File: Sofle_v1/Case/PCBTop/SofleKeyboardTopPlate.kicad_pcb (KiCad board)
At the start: 2 copper layers, 137.2 x 109.2 mm, 5 parts

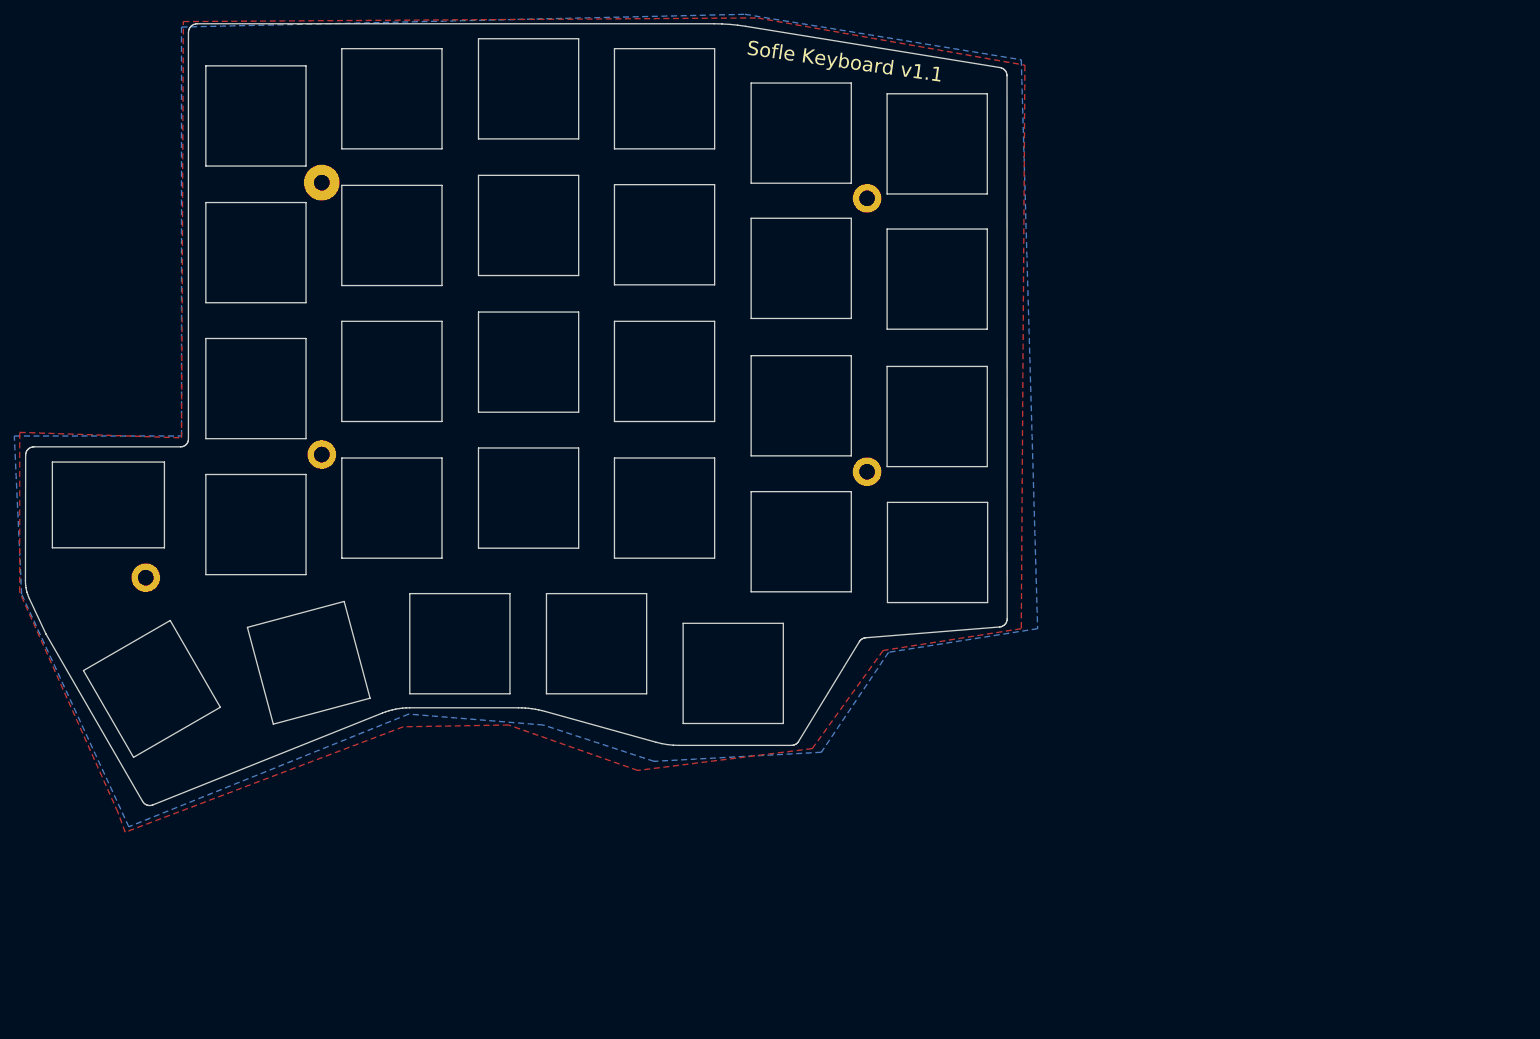
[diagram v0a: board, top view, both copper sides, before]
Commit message: Plates.
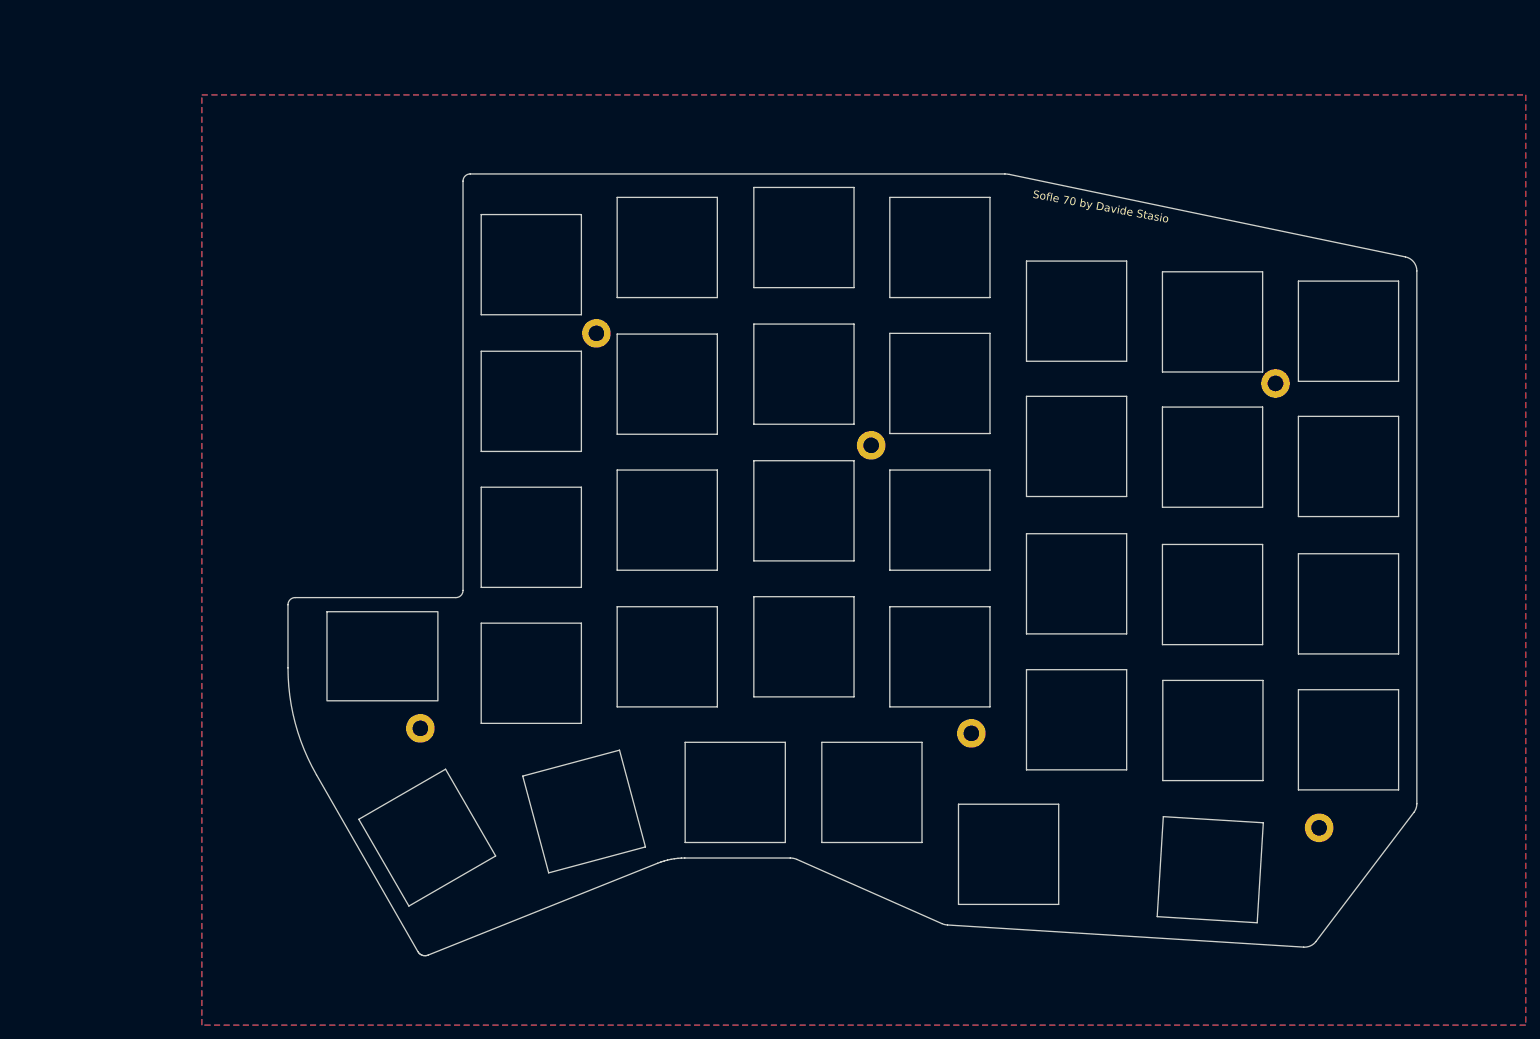
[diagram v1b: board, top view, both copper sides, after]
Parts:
- removed ? (x5): , Wire_Pads:SolderWirePad_single_0-8mmDrill
- added SW1: SW_PUSH, SofleKeyboard:CherryMX_KailhLowProfile_Hotswap_Top-Plate, F.Cu at (91.0, 50.2)
- added SW10: SW_PUSH, SofleKeyboard:CherryMX_KailhLowProfile_Hotswap_Top-Plate, F.Cu at (148.1, 66.8)
- added SW11: SW_PUSH, SofleKeyboard:CherryMX_KailhLowProfile_Hotswap_Top-Plate, F.Cu at (167.2, 75.6)
- added SW12: SW_PUSH, SofleKeyboard:CherryMX_KailhLowProfile_Hotswap_Top-Plate, F.Cu at (186.2, 77.1)
- added SW13: SW_PUSH, SofleKeyboard:CherryMX_KailhLowProfile_Hotswap_Top-Plate, F.Cu at (91.0, 88.3)
- added SW14: SW_PUSH, SofleKeyboard:CherryMX_KailhLowProfile_Hotswap_Top-Plate, F.Cu at (110.0, 85.9)
- added SW15: SW_PUSH, SofleKeyboard:CherryMX_KailhLowProfile_Hotswap_Top-Plate, F.Cu at (129.1, 84.6)
- added SW16: SW_PUSH, SofleKeyboard:CherryMX_KailhLowProfile_Hotswap_Top-Plate, F.Cu at (148.1, 85.9)
- added SW17: SW_PUSH, SofleKeyboard:CherryMX_KailhLowProfile_Hotswap_Top-Plate, F.Cu at (167.2, 94.8)
- added SW18: SW_PUSH, SofleKeyboard:CherryMX_KailhLowProfile_Hotswap_Top-Plate, F.Cu at (186.2, 96.3)
- added SW19: SW_PUSH, SofleKeyboard:CherryMX_KailhLowProfile_Hotswap_Top-Plate, F.Cu at (91.0, 107.3)
- added SW2: SW_PUSH, SofleKeyboard:CherryMX_KailhLowProfile_Hotswap_Top-Plate, F.Cu at (110.0, 47.8)
- added SW20: SW_PUSH, SofleKeyboard:CherryMX_KailhLowProfile_Hotswap_Top-Plate, F.Cu at (110.0, 105.0)
- added SW21: SW_PUSH, SofleKeyboard:CherryMX_KailhLowProfile_Hotswap_Top-Plate, F.Cu at (129.1, 103.6)
- added SW22: SW_PUSH, SofleKeyboard:CherryMX_KailhLowProfile_Hotswap_Top-Plate, F.Cu at (148.1, 105.0)
- added SW23: SW_PUSH, SofleKeyboard:CherryMX_KailhLowProfile_Hotswap_Top-Plate, F.Cu at (167.2, 113.8)
- added SW24: SW_PUSH, SofleKeyboard:CherryMX_KailhLowProfile_Hotswap_Top-Plate, F.Cu at (186.3, 115.3)
- added SW25: Rotary_Encoder_Switch, SofleKeyboard:RotaryEncoder_Alps_EC11E-Switch_Vertical_H20mm-keebio_Top-Plate, F.Cu at (70.5, 104.7)
- added SW26: SW_PUSH, SofleKeyboard:CherryMX_KailhLowProfile_Hotswap_Top-Plate, F.Cu at (76.5, 130.3)
- added SW27: SW_PUSH, SofleKeyboard:CherryMX_KailhLowProfile_Hotswap_Top-Plate, F.Cu at (98.4, 126.6)
- added SW28: SW_PUSH, SofleKeyboard:CherryMX_KailhLowProfile_Hotswap_Top-Plate, F.Cu at (119.5, 124.0)
- added SW29: SW_PUSH, SofleKeyboard:CherryMX_KailhLowProfile_Hotswap_Top-Plate, F.Cu at (138.6, 124.0)
- added SW3: SW_PUSH, SofleKeyboard:CherryMX_KailhLowProfile_Hotswap_Top-Plate, F.Cu at (129.1, 46.4)
- added SW30: SW_PUSH, SofleKeyboard:CherryMX_KailhLowProfile_Hotswap_Top-Plate, F.Cu at (157.7, 132.6)
- added SW31: SW_PUSH, SofleKeyboard:CherryMX_KailhLowProfile_Hotswap_Top-Plate, F.Cu at (205.2, 59.5)
- added SW32: SW_PUSH, SofleKeyboard:CherryMX_KailhLowProfile_Hotswap_Top-Plate, F.Cu at (205.2, 78.4)
- added SW33: SW_PUSH, SofleKeyboard:CherryMX_KailhLowProfile_Hotswap_Top-Plate, F.Cu at (205.2, 97.6)
- added SW34: SW_PUSH, SofleKeyboard:CherryMX_KailhLowProfile_Hotswap_Top-Plate, F.Cu at (205.2, 116.6)
- added SW35: SW_PUSH, SofleKeyboard:CherryMX_KailhLowProfile_Hotswap_Top-Plate, F.Cu at (185.9, 134.8)
- added SW4: SW_PUSH, SofleKeyboard:CherryMX_KailhLowProfile_Hotswap_Top-Plate, F.Cu at (148.1, 47.8)
- added SW5: SW_PUSH, SofleKeyboard:CherryMX_KailhLowProfile_Hotswap_Top-Plate, F.Cu at (167.2, 56.7)
- added SW6: SW_PUSH, SofleKeyboard:CherryMX_KailhLowProfile_Hotswap_Top-Plate, F.Cu at (186.2, 58.2)
- added SW7: SW_PUSH, SofleKeyboard:CherryMX_KailhLowProfile_Hotswap_Top-Plate, F.Cu at (91.0, 69.3)
- added SW8: SW_PUSH, SofleKeyboard:CherryMX_KailhLowProfile_Hotswap_Top-Plate, F.Cu at (110.0, 66.9)
- added SW9: SW_PUSH, SofleKeyboard:CherryMX_KailhLowProfile_Hotswap_Top-Plate, F.Cu at (129.1, 65.5)
- added TH3: HOLE, SofleKeyboard:SolderWirePad_single_0-8mmDrill, F.Cu at (100.1, 59.8)
- added TH4: HOLE, SofleKeyboard:SolderWirePad_single_0-8mmDrill, F.Cu at (195.0, 66.8)
- added TH5: HOLE, SofleKeyboard:SolderWirePad_single_0-8mmDrill, F.Cu at (138.5, 75.5)
- added TH6: HOLE, SofleKeyboard:SolderWirePad_single_0-8mmDrill, F.Cu at (201.1, 128.9)
- added TH7: HOLE, SofleKeyboard:SolderWirePad_single_0-8mmDrill, F.Cu at (75.5, 115.0)
- added TH8: HOLE, SofleKeyboard:SolderWirePad_single_0-8mmDrill, F.Cu at (152.5, 115.7)
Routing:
- added copper zone on B.Cu, net GND
- added copper zone on F.Cu, net GND
- removed copper zone on B.Cu, net (none)
- removed copper zone on F.Cu, net (none)
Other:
- board size 137.2 x 109.2 mm -> 157.7 x 109.2 mm
- net class Default removed
- board text added: "Sofle 70 by Davide Stasio"
- board text removed: "Sofle Keyboard v1.1"
